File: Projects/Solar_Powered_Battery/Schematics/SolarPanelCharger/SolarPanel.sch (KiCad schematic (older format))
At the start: 3 parts

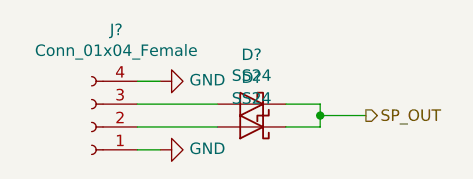
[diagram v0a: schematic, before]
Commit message: update solar panel schematic
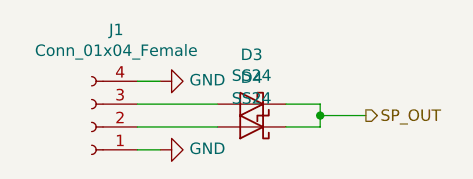
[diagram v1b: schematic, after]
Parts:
- D3, D4: renamed from D?; footprint (none) -> custom-footprints:SMB_DO-214AA
- J1: renamed from J?; footprint (none) -> TerminalBlock_Phoenix:TerminalBlock_Phoenix_MKDS-1,5-4_1x04_P5.00mm_Horizontal
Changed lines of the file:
@@
 EESchema Schematic File Version 4
+LIBS:SolarPanelCharger-cache
 EELAYER 29 0
 EELAYER END
 $Descr A4 11693 8268
 encoding utf-8
-Sheet 2 3
+Sheet 2 6
 Title ""
 Date ""
@@
 $EndDescr
 $Comp
-L Connector:Conn_01x04_Female J?
+L Connector:Conn_01x04_Female J1
 U 1 1 5CB1C1A6
 P 2250 2250
-F 0 "J?" H 2142 1825 50  0000 C CNN
+F 0 "J1" H 2142 1825 50  0000 C CNN
 F 1 "Conn_01x04_Female" H 2142 1916 50  0000 C CNN
-F 2 "" H 2250 2250 50  0001 C CNN
+F 2 "TerminalBlock_Phoenix:TerminalBlock_Phoenix_MKDS-1,5-4_1x04_P5.00mm_Horizontal" H 2250 2250 50  0001 C CNN
 F 3 "~" H 2250 2250 50  0001 C CNN
 	1    2250 2250
@@
 $EndComp
 $Comp
-L Device:D_Schottky D?
+L Device:D_Schottky D3
 U 1 1 5CB1EC75
 P 2950 2150
-F 0 "D?" H 2950 1934 50  0000 C CNN
+F 0 "D3" H 2950 1934 50  0000 C CNN
 F 1 "SS24" H 2950 2025 50  0000 C CNN
-F 2 "" H 2950 2150 50  0001 C CNN
+F 2 "custom-footprints:SMB_DO-214AA" H 2950 2150 50  0001 C CNN
 F 3 "~" H 2950 2150 50  0001 C CNN
 	1    2950 2150
@@
 $EndComp
 $Comp
-L Device:D_Schottky D?
+L Device:D_Schottky D4
 U 1 1 5CB1F886
 P 2950 2250
-F 0 "D?" H 2950 2034 50  0000 C CNN
+F 0 "D4" H 2950 2034 50  0000 C CNN
 F 1 "SS24" H 2950 2125 50  0000 C CNN
-F 2 "" H 2950 2250 50  0001 C CNN
+F 2 "custom-footprints:SMB_DO-214AA" H 2950 2250 50  0001 C CNN
 F 3 "~" H 2950 2250 50  0001 C CNN
 	1    2950 2250
@@
 $EndComp
 $Comp
-L power:GND #PWR?
+L power:GND #PWR09
 U 1 1 5CB2015B
 P 2550 2050
-F 0 "#PWR?" H 2550 1800 50  0001 C CNN
+F 0 "#PWR09" H 2550 1800 50  0001 C CNN
 F 1 "GND" V 2555 1922 50  0000 R CNN
 F 2 "" H 2550 2050 50  0001 C CNN
@@
 	2450 2050 2550 2050
 $Comp
-L power:GND #PWR?
+L power:GND #PWR010
 U 1 1 5CB21365
 P 2550 2350
-F 0 "#PWR?" H 2550 2100 50  0001 C CNN
+F 0 "#PWR010" H 2550 2100 50  0001 C CNN
 F 1 "GND" V 2555 2222 50  0000 R CNN
 F 2 "" H 2550 2350 50  0001 C CNN
